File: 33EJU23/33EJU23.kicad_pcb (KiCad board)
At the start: 2 copper layers, 54 x 85.7 mm, 110 parts, among them CN1 HDMI, J1 VGA, J10 Conn_01x02, J11 Conn_01x03, J12 VIDEO, J13 Conn_02x05_Odd_Even, J2 EXT, J3 JOY-1, J4 USB_A, J5 USB_A, J6 USB_A, J7 Conn_01x04_Male, J8 Conn_01x20, J9 Conn_01x12, Q1 BC850, U1 FE1.1s, U2 MW7211A, U3 XN297L, U4 CXA1645M, Y1 12MHz, Y2 12MHz, Y3 16MHz, Y4 16MHz, Y5 4,43M*, Y5_2 12MHz

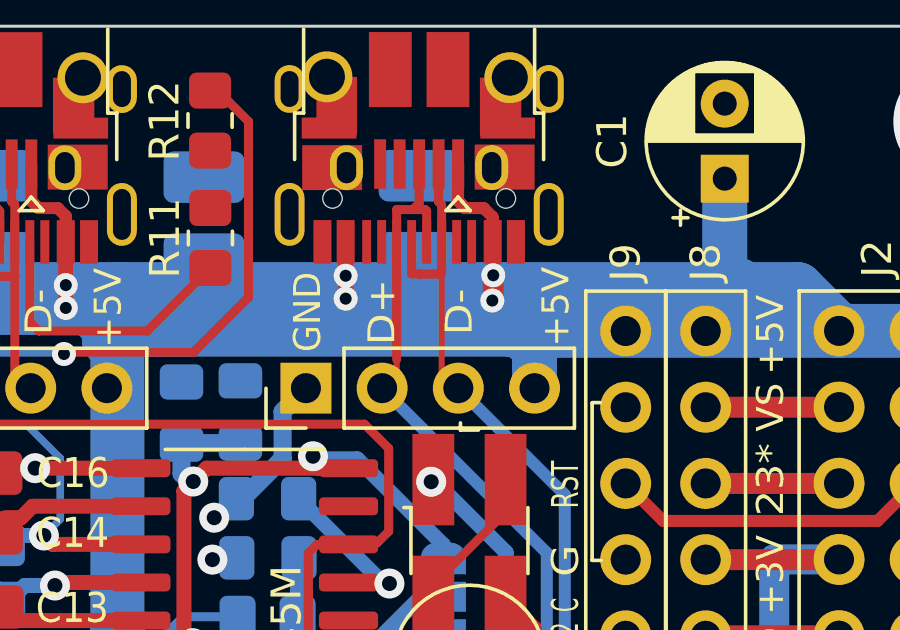
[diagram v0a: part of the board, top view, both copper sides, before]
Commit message: create
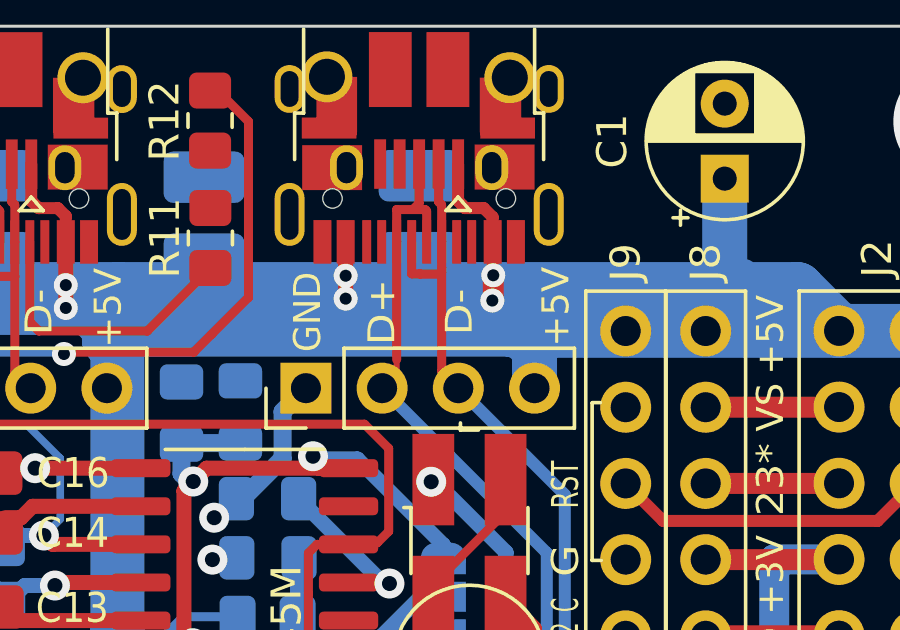
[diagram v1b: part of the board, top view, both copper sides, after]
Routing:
- net /D-: track 41.8 -> 45.3 mm
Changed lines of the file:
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@@
     (property "Sheetfile" "33EJU23.kicad_sch")
     (property "Sheetname" "")
-    (attr smd)
+    (attr through_hole)
     (fp_text reference "J3" (at 7.7724 0.0283 90) (layer "F.SilkS")
       (effects (font (size 1 1) (thickness 0.15)))
@@
   (segment (start 46.228 38.862) (end 46.285 38.805) (width 0.3) (layer "B.Cu") (net 59))
   (segment (start 62.5896 35.127) (end 62.5896 36.195) (width 0.3) (layer "F.Cu") (net 61))
-  (segment (start 63.5896 39.4496) (end 64.145 40.005) (width 0.2) (layer "F.Cu") (net 61))
+  (segment (start 63.5896 35.127) (end 63.5896 35.9784) (width 0.3) (layer "F.Cu") (net 61))
+  (segment (start 63.5896 35.9784) (end 63.5896 39.4496) (width 0.3) (layer "F.Cu") (net 61))
   (segment (start 62.865 36.195) (end 62.5896 36.195) (width 0.3) (layer "F.Cu") (net 61))
-  (segment (start 63.5896 35.127) (end 63.5896 36.152) (width 0.3) (layer "F.Cu") (net 61))
   (segment (start 63.5896 36.152) (end 63.5896 39.4496) (width 0.2) (layer "F.Cu") (net 61))
   (segment (start 63.5896 33.894893) (end 63.5896 35.127) (width 0.3) (layer "F.Cu") (net 61))
   (segment (start 63.5396 36.202) (end 62.872 36.202) (width 0.3) (layer "F.Cu") (net 61))
+  (segment (start 63.5896 39.4496) (end 64.145 40.005) (width 0.3) (layer "F.Cu") (net 61))
   (segment (start 63.487945 33.793238) (end 63.5896 33.894893) (width 0.3) (layer "F.Cu") (net 61))
   (segment (start 63.5896 36.152) (end 63.5396 36.202) (width 0.3) (layer "F.Cu") (net 61))
   (segment (start 63.487945 32.534506) (end 63.487945 33.793238) (width 0.3) (layer "F.Cu") (net 61))
+  (segment (start 63.5896 35.9784) (end 63.5896 36.152) (width 0.3) (layer "F.Cu") (net 61))
   (segment (start 62.872 36.202) (end 62.865 36.195) (width 0.3) (layer "F.Cu") (net 61))
   (segment (start 62.354207 67.945) (end 67.691 62.608207) (width 0.4) (layer "B.Cu") (net 61))
